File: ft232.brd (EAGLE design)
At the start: 47.9 x 36.8 mm, 12 parts, among them U1 FT232RL-BASICSSOP

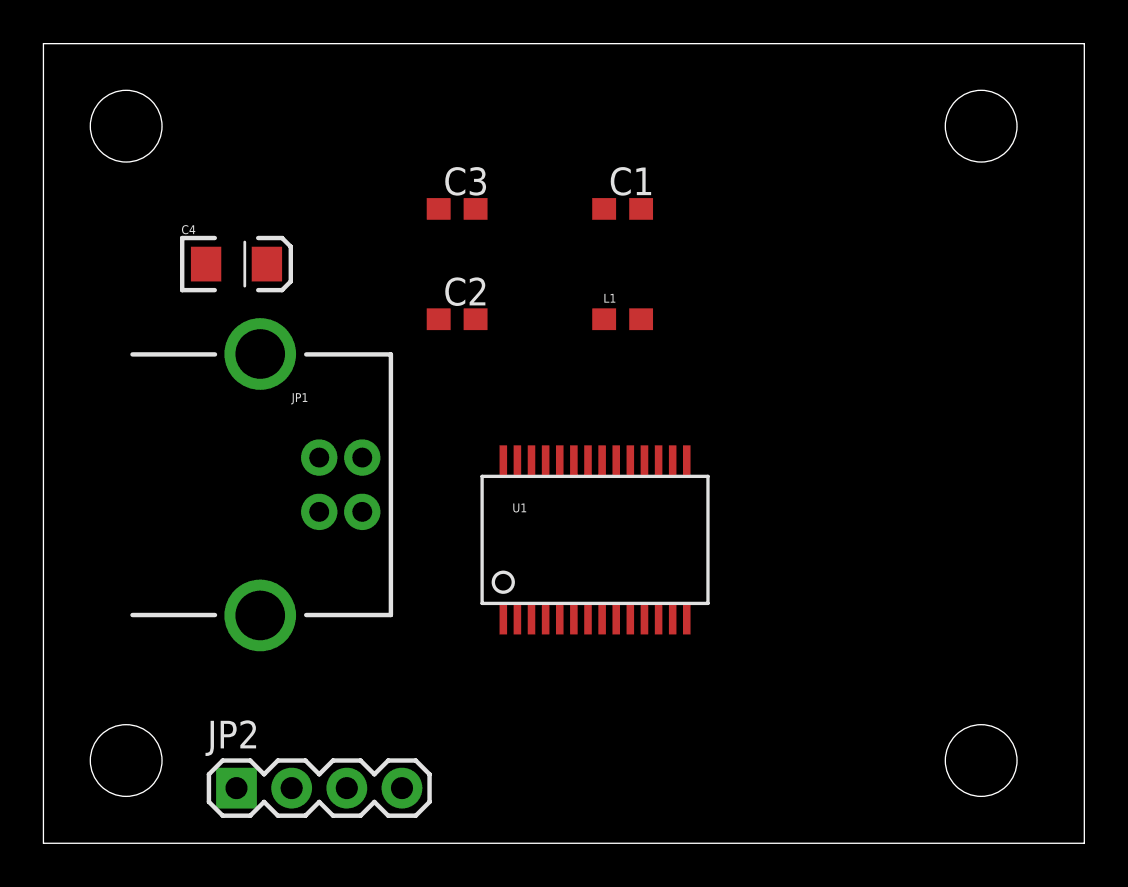
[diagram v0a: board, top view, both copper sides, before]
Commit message: Added CAM files
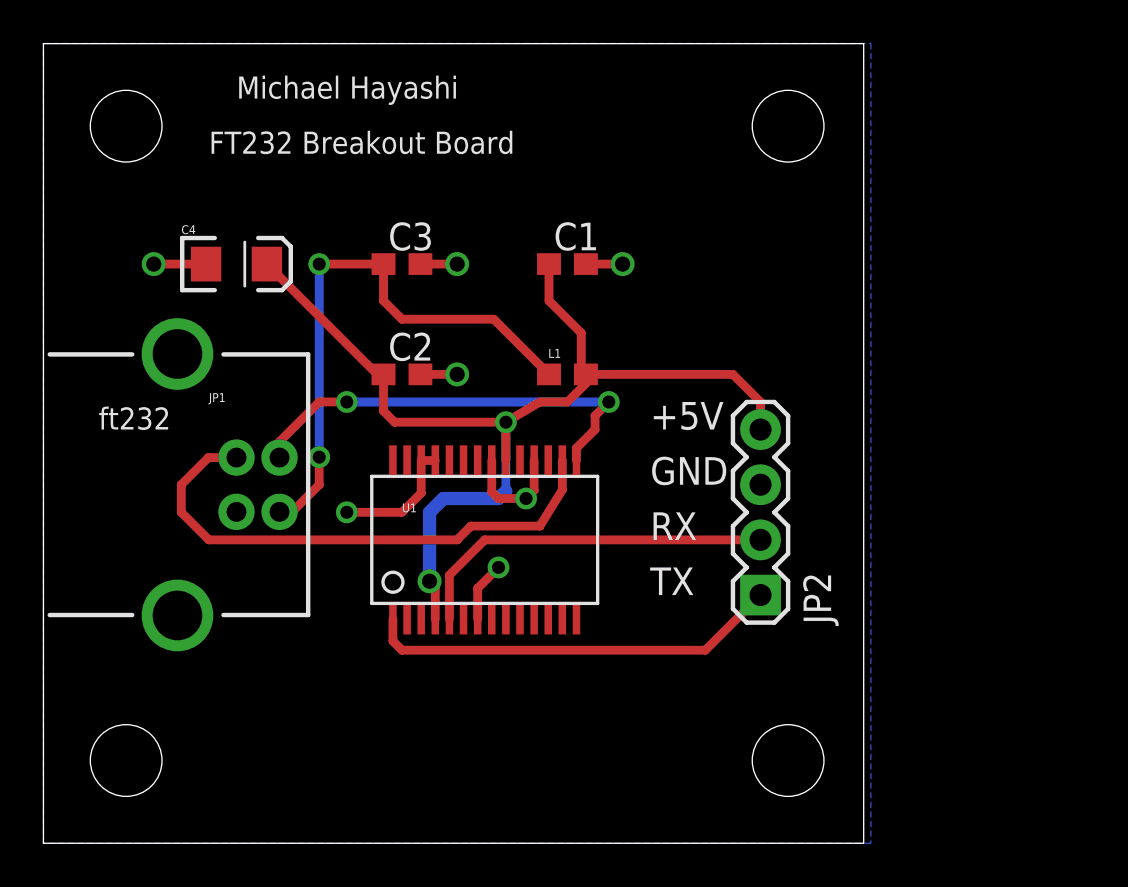
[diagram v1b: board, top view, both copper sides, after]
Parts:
- moved JP2 25.7 mm to (33.0, 11.4), turned to 90 degrees
- moved STANDOFF3 8.89 mm to (34.3, 33.0)
- moved STANDOFF4 8.89 mm to (34.3, 3.81)
- moved U1 5.08 mm to (20.3, 14.0)
- moved JP1 3.81 mm to (8.89, 16.5)
- moved C1 3.59 mm to (24.1, 26.7)
- moved L1 3.59 mm to (24.1, 21.6)
- moved C2 3.59 mm to (16.5, 21.6)
- moved C3 3.59 mm to (16.5, 26.7)
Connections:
- net GND: now also JP1.GND
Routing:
- net +5V: track 0.00 -> 49.2 mm, vias 0 -> 2
- net N$1: track 0.00 -> 26.2 mm, vias 0 -> 2
- net N$3: track 0.00 -> 24.9 mm
- net GND: track 0.00 -> 21.3 mm, vias 0 -> 7
- net N$4: track 0.00 -> 20.0 mm, vias 0 -> 2
- net TX: track 0.00 -> 19.2 mm
- net RX: track 0.00 -> 17.0 mm
- added copper zone on layer 16, net GND
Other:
- board size 47.9 x 36.8 mm -> 37.8 x 36.8 mm
- board text added: "+5V"
- board text added: ">DRAWING_NAME"
- board text added: ">LAST_DATE_TIME"
- board text added: "FT232 Breakout Board"
- board text added: "GND"
- board text added: "Michael Hayashi"
- board text added: "RX"
- board text added: "TX"
